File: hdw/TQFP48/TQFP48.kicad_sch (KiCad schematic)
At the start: 3 parts, among them J1 Conn_01x24, J2 Conn_01x24, U1 TQFP48

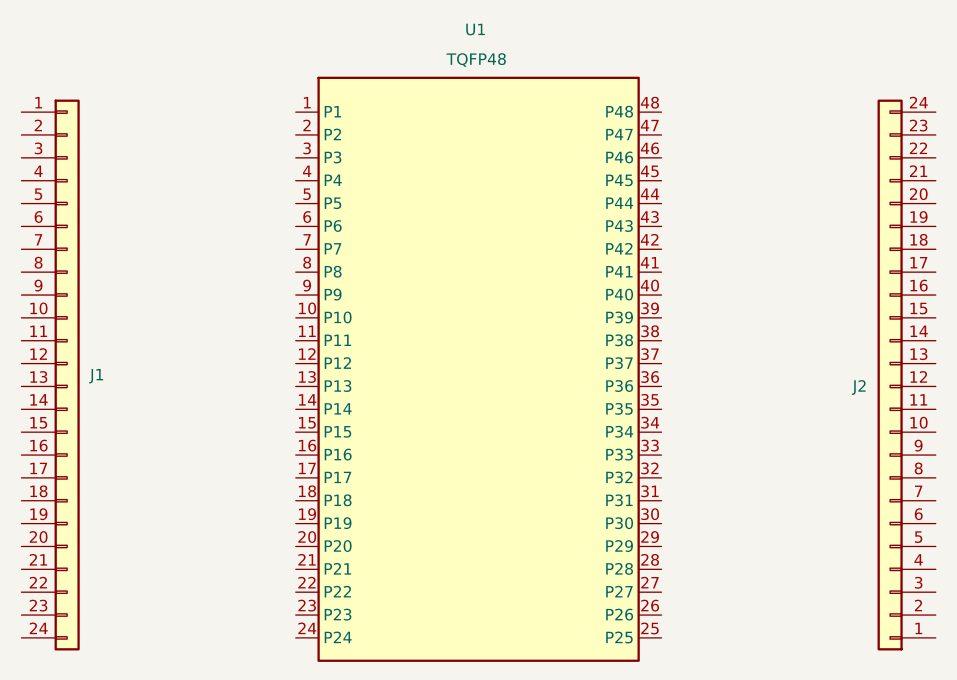
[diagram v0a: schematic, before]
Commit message: Save changes at: 1748186389
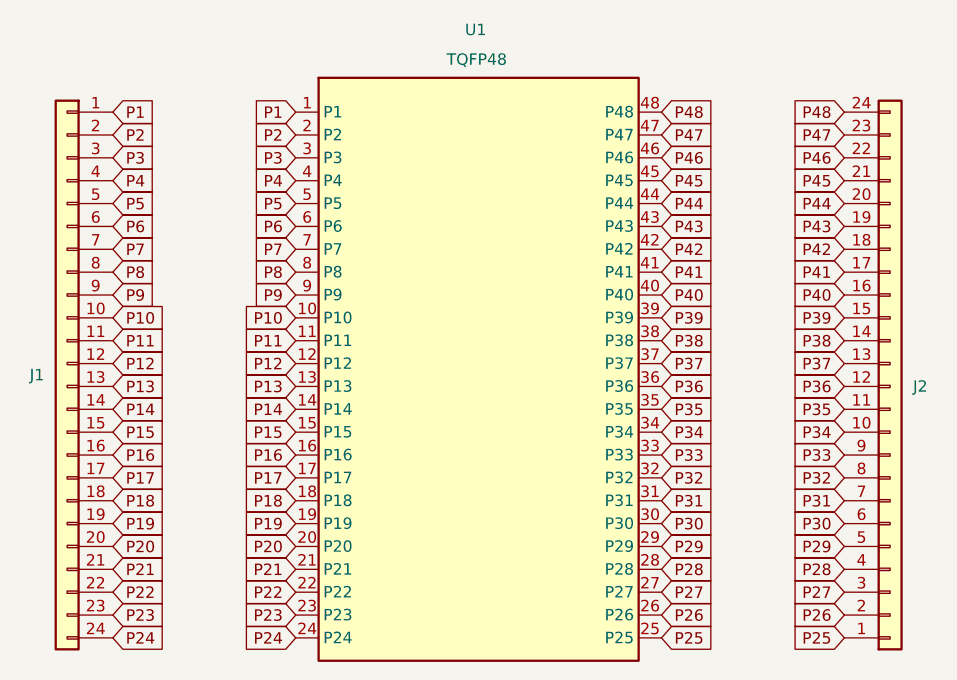
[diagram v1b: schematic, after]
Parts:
- J1, J2: footprint (none) -> Connector_PinHeader_2.54mm:PinHeader_1x24_P2.54mm_Vertical
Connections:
- net P1: now reaches U1.1 (P1)
- net P1: now also J1.1 (Pin_1)
- net P10: now reaches U1.10 (P10)
- net P10: now also J1.10 (Pin_10)
- net P11: now reaches U1.11 (P11)
- net P11: now also J1.11 (Pin_11)
- net P12: now reaches U1.12 (P12)
- net P12: now also J1.12 (Pin_12)
- net P13: now reaches U1.13 (P13)
- net P13: now also J1.13 (Pin_13)
- net P14: now reaches U1.14 (P14)
- net P14: now also J1.14 (Pin_14)
- net P15: now reaches U1.15 (P15)
- net P15: now also J1.15 (Pin_15)
- net P16: now reaches U1.16 (P16)
- net P16: now also J1.16 (Pin_16)
- net P17: now reaches U1.17 (P17)
- net P17: now also J1.17 (Pin_17)
- net P18: now reaches U1.18 (P18)
- net P18: now also J1.18 (Pin_18)
- net P19: now reaches U1.19 (P19)
- net P19: now also J1.19 (Pin_19)
- net P2: now reaches U1.2 (P2)
- net P2: now also J1.2 (Pin_2)
- net P20: now reaches U1.20 (P20)
- net P20: now also J1.20 (Pin_20)
- net P21: now reaches U1.21 (P21)
- net P21: now also J1.21 (Pin_21)
- net P22: now reaches U1.22 (P22)
- net P22: now also J1.22 (Pin_22)
- net P23: now reaches U1.23 (P23)
- net P23: now also J1.23 (Pin_23)
- net P24: now reaches U1.24 (P24)
- net P24: now also J1.24 (Pin_24)
- net P25: now reaches U1.25 (P25)
- net P25: now also J2.1 (Pin_1)
- net P26: now reaches U1.26 (P26)
- net P26: now also J2.2 (Pin_2)
- net P27: now reaches U1.27 (P27)
- net P27: now also J2.3 (Pin_3)
- net P28: now reaches U1.28 (P28)
- net P28: now also J2.4 (Pin_4)
- net P29: now reaches U1.29 (P29)
- net P29: now also J2.5 (Pin_5)
- net P3: now reaches U1.3 (P3)
- net P3: now also J1.3 (Pin_3)
- net P30: now reaches U1.30 (P30)
- net P30: now also J2.6 (Pin_6)
- net P31: now reaches U1.31 (P31)
- net P31: now also J2.7 (Pin_7)
- net P32: now reaches U1.32 (P32)
- net P32: now also J2.8 (Pin_8)
- net P33: now reaches U1.33 (P33)
- net P33: now also J2.9 (Pin_9)
- net P34: now reaches U1.34 (P34)
- net P34: now also J2.10 (Pin_10)
- net P35: now reaches U1.35 (P35)
- net P35: now also J2.11 (Pin_11)
- net P36: now reaches U1.36 (P36)
- net P36: now also J2.12 (Pin_12)
- net P37: now reaches U1.37 (P37)
- net P37: now also J2.13 (Pin_13)
- net P38: now reaches U1.38 (P38)
- net P38: now also J2.14 (Pin_14)
- net P39: now reaches U1.39 (P39)
- net P39: now also J2.15 (Pin_15)
- net P4: now reaches U1.4 (P4)
- net P4: now also J1.4 (Pin_4)
- net P40: now reaches U1.40 (P40)
- net P40: now also J2.16 (Pin_16)
- net P41: now reaches U1.41 (P41)
- net P41: now also J2.17 (Pin_17)
- net P42: now reaches U1.42 (P42)
- net P42: now also J2.18 (Pin_18)
- net P43: now reaches U1.43 (P43)
- net P43: now also J2.19 (Pin_19)
- net P44: now reaches U1.44 (P44)
- net P44: now also J2.20 (Pin_20)
- net P45: now reaches U1.45 (P45)
- net P45: now also J2.21 (Pin_21)
- net P46: now reaches U1.46 (P46)
- net P46: now also J2.22 (Pin_22)
- net P47: now reaches U1.47 (P47)
- net P47: now also J2.23 (Pin_23)
- net P48: now reaches U1.48 (P48)
- net P48: now also J2.24 (Pin_24)
- net P5: now reaches U1.5 (P5)
- net P5: now also J1.5 (Pin_5)
- net P6: now reaches U1.6 (P6)
- net P6: now also J1.6 (Pin_6)
- net P7: now reaches U1.7 (P7)
- net P7: now also J1.7 (Pin_7)
- net P8: now reaches U1.8 (P8)
- net P8: now also J1.8 (Pin_8)
- net P9: now reaches U1.9 (P9)
- net P9: now also J1.9 (Pin_9)
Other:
- moved on the sheet: J1, J2
